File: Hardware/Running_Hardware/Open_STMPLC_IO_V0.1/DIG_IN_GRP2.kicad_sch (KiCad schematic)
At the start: 54 parts, among them J16 Screw_Terminal_01x02, J17 Screw_Terminal_01x02, J18 Screw_Terminal_01x02, J19 Screw_Terminal_01x02, J20 Screw_Terminal_01x02, J3 Screw_Terminal_01x02, U12 6N137, U20 6N137, U21 6N137, U22 6N137, U23 6N137, U24 6N137

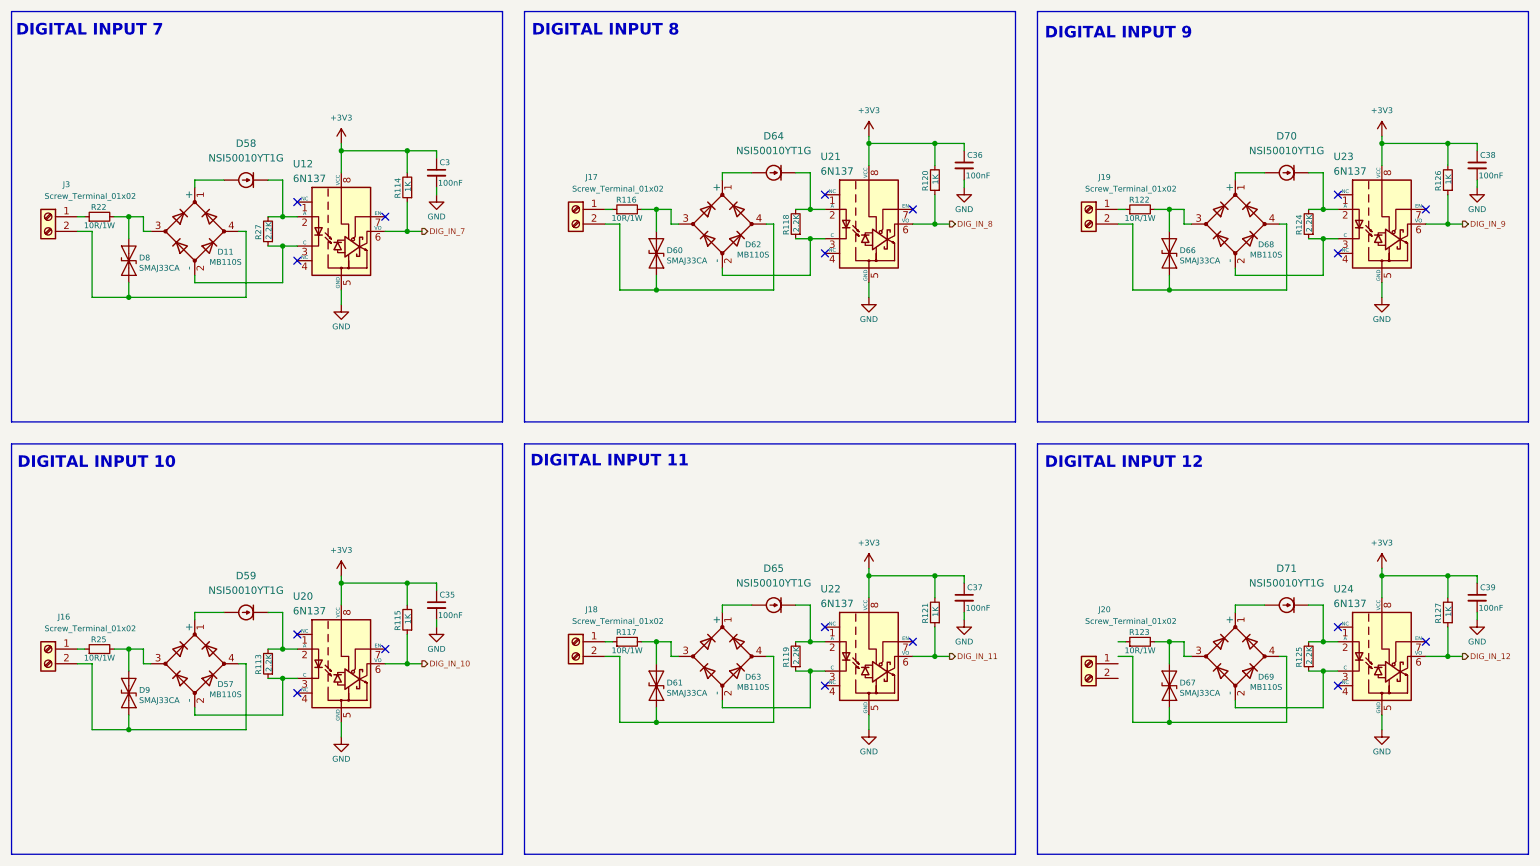
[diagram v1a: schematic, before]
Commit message: Analog input section
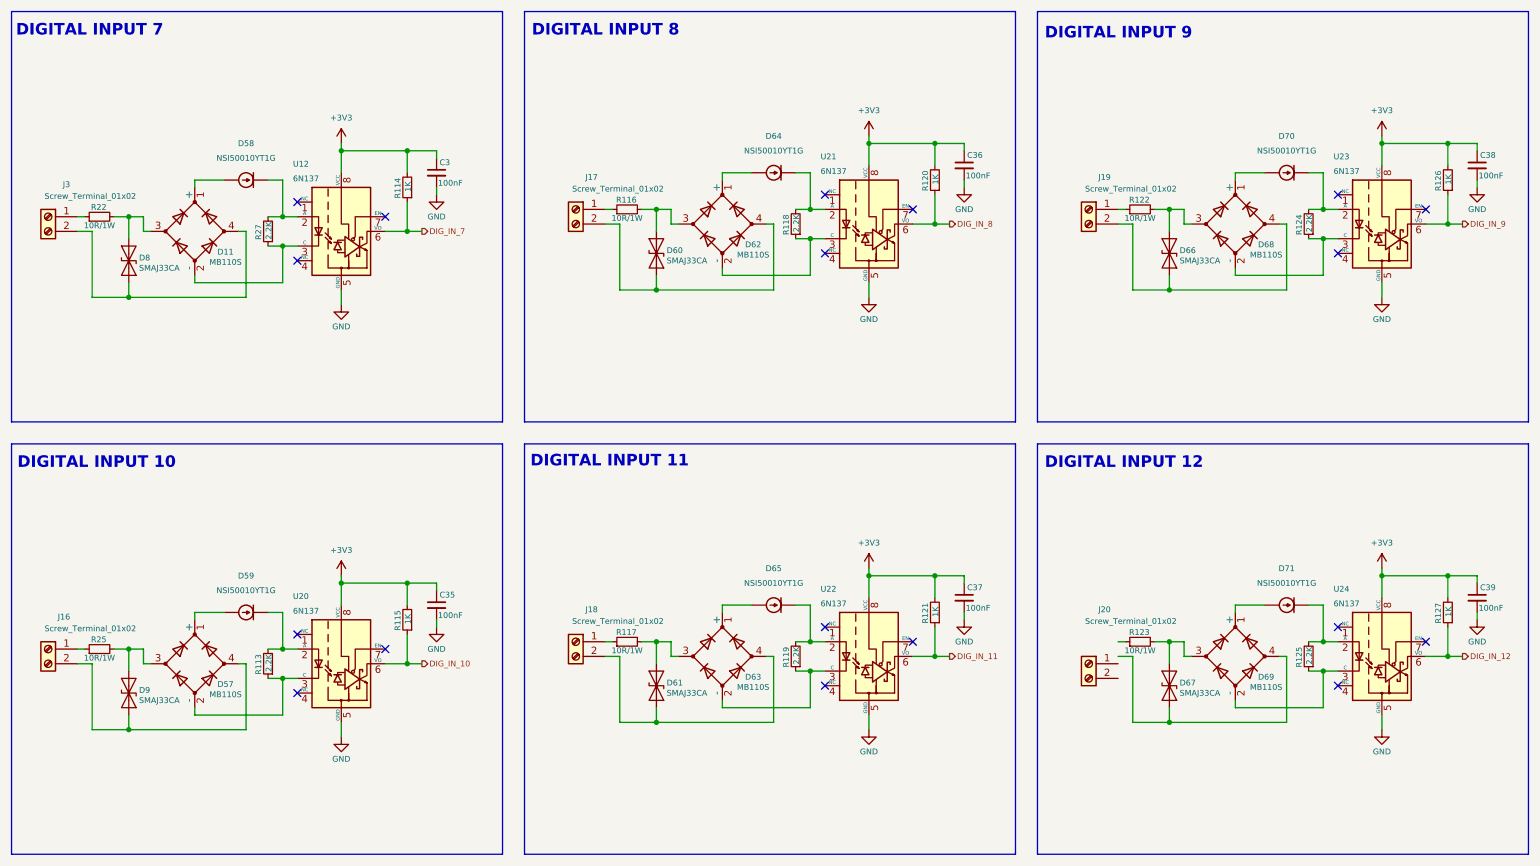
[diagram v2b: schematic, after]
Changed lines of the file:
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@@
 			(effects
 				(font
-					(size 1.27 1.27)
+					(size 1 1)
 				)
 				(justify left)
@@
 			(effects
 				(font
-					(size 1.27 1.27)
+					(size 1 1)
 				)
 				(justify left)
@@
 			(effects
 				(font
-					(size 1.27 1.27)
+					(size 1 1)
 				)
 			)
@@
 			(effects
 				(font
-					(size 1.27 1.27)
+					(size 1 1)
 				)
 			)
@@
 			(effects
 				(font
-					(size 1.27 1.27)
+					(size 1 1)
 				)
 			)
@@
 			(effects
 				(font
-					(size 1.27 1.27)
+					(size 1 1)
 				)
 			)
@@
 			(effects
 				(font
-					(size 1.27 1.27)
+					(size 1 1)
 				)
 			)
@@
 			(effects
 				(font
-					(size 1.27 1.27)
+					(size 1 1)
 				)
 			)
@@
 			(effects
 				(font
-					(size 1.27 1.27)
+					(size 1 1)
 				)
 				(justify left)
@@
 			(effects
 				(font
-					(size 1.27 1.27)
+					(size 1 1)
 				)
 				(justify left)
@@
 			(effects
 				(font
-					(size 1.27 1.27)
+					(size 1 1)
 				)
 			)
@@
 			(effects
 				(font
-					(size 1.27 1.27)
+					(size 1 1)
 				)
 			)
@@
 			(effects
 				(font
-					(size 1.27 1.27)
+					(size 1 1)
 				)
 				(justify left)
@@
 			(effects
 				(font
-					(size 1.27 1.27)
+					(size 1 1)
 				)
 				(justify left)
@@
 			(effects
 				(font
-					(size 1.27 1.27)
+					(size 1 1)
 				)
 				(justify left)
@@
 			(effects
 				(font
-					(size 1.27 1.27)
+					(size 1 1)
 				)
 				(justify left)
@@
 			(effects
 				(font
-					(size 1.27 1.27)
+					(size 1 1)
 				)
 				(justify left)
@@
 			(effects
 				(font
-					(size 1.27 1.27)
+					(size 1 1)
 				)
 				(justify left)
@@
 			(effects
 				(font
-					(size 1.27 1.27)
+					(size 1 1)
 				)
 			)
@@
 			(effects
 				(font
-					(size 1.27 1.27)
+					(size 1 1)
 				)
 			)
@@
 			(effects
 				(font
-					(size 1.27 1.27)
+					(size 1 1)
 				)
 				(justify left)
@@
 			(effects
 				(font
-					(size 1.27 1.27)
+					(size 1 1)
 				)
 				(justify left)
@@
 			(effects
 				(font
-					(size 1.27 1.27)
+					(size 1 1)
 				)
 			)
@@
 			(effects
 				(font
-					(size 1.27 1.27)
+					(size 1 1)
 				)
 			)
